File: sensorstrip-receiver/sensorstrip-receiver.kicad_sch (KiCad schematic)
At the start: 6 parts, among them J1 Conn_01x02_MountingPin, J2 Conn_01x02_MountingPin

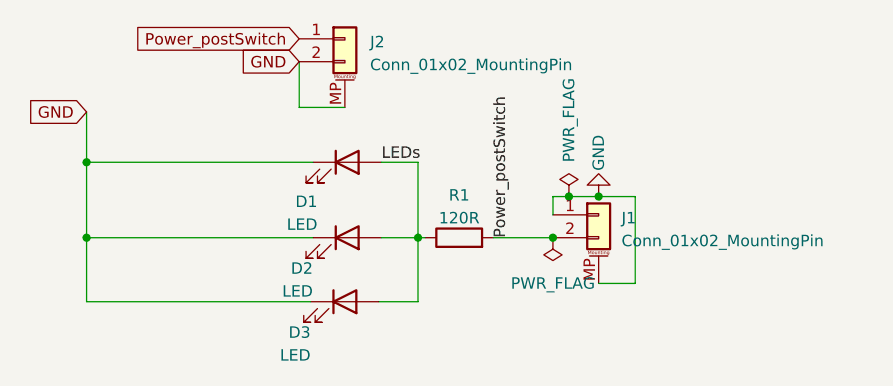
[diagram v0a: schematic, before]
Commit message: fix humongous oversight
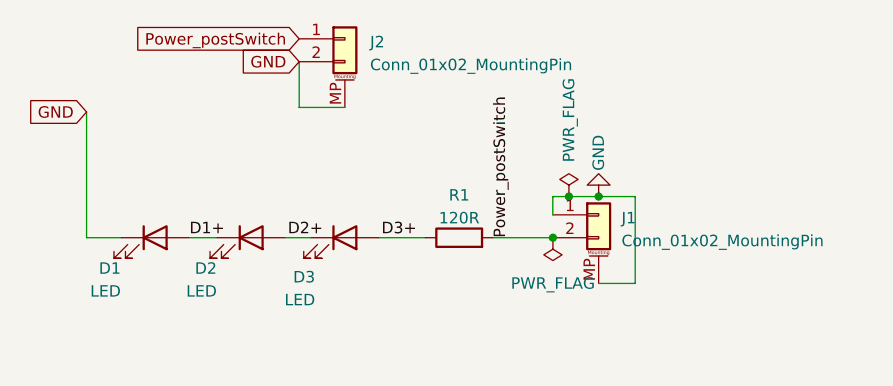
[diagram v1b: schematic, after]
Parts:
- renumbered D3 to D1, D1 to D3
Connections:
- net GND: no longer D2.1 (K), D3.1 (K)
- net LEDs renamed D3+
- net D3+: no longer D1.2 (A), D2.2 (A)
- new net D1+: D1.2 (A), D2.1 (K)
- new net D2+: D2.2 (A), D3.1 (K)
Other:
- moved on the sheet: D1, D2, D3
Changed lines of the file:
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@@
   (junction (at 117.348 86.868) (diameter 0) (color 0 0 0 0)
   )
-  (junction (at 63.754 83.058) (diameter 0) (color 0 0 0 0)
-  )
-  (junction (at 100.584 91.44) (diameter 0) (color 0 0 0 0)
-  )
-  (junction (at 63.754 91.44) (diameter 0) (color 0 0 0 0)
-  )
   (junction (at 120.65 86.868) (diameter 0) (color 0 0 0 0)
   )
   (junction (at 115.57 91.44) (diameter 0) (color 0 0 0 0)
   )
-  (wire (pts (xy 88.9 91.44) (xy 63.754 91.44))
-    (stroke (width 0) (type default) (color 0 0 0 0))
-  )
-  (wire (pts (xy 63.754 83.058) (xy 63.754 77.47))
-    (stroke (width 0) (type default) (color 0 0 0 0))
-  )
-  (wire (pts (xy 100.584 98.552) (xy 96.266 98.552))
+  (wire (pts (xy 78.232 91.44) (xy 75.184 91.44))
     (stroke (width 0) (type default) (color 0 0 0 0))
   )
@@
     (stroke (width 0) (type default) (color 0 0 0 0))
   )
-  (wire (pts (xy 63.754 91.44) (xy 63.754 98.552))
-    (stroke (width 0) (type default) (color 0 0 0 0))
-  )
   (wire (pts (xy 120.65 86.868) (xy 117.348 86.868))
     (stroke (width 0) (type default) (color 0 0 0 0))
@@
     (stroke (width 0) (type default) (color 0 0 0 0))
   )
-  (wire (pts (xy 101.346 91.44) (xy 100.584 91.44))
-    (stroke (width 0) (type default) (color 0 0 0 0))
-  )
-  (wire (pts (xy 88.646 98.552) (xy 63.754 98.552))
-    (stroke (width 0) (type default) (color 0 0 0 0))
-  )
-  (wire (pts (xy 63.754 83.058) (xy 63.754 91.44))
-    (stroke (width 0) (type default) (color 0 0 0 0))
-  )
-  (wire (pts (xy 100.584 83.058) (xy 96.52 83.058))
-    (stroke (width 0) (type default) (color 0 0 0 0))
-  )
-  (wire (pts (xy 100.584 91.44) (xy 100.584 83.058))
+  (wire (pts (xy 67.564 91.44) (xy 63.754 91.44))
+    (stroke (width 0) (type default) (color 0 0 0 0))
+  )
+  (wire (pts (xy 63.754 77.47) (xy 63.754 91.44))
+    (stroke (width 0) (type default) (color 0 0 0 0))
+  )
+  (wire (pts (xy 88.646 91.44) (xy 85.852 91.44))
     (stroke (width 0) (type default) (color 0 0 0 0))
   )
@@
     (stroke (width 0) (type default) (color 0 0 0 0))
   )
-  (wire (pts (xy 88.9 83.058) (xy 63.754 83.058))
-    (stroke (width 0) (type default) (color 0 0 0 0))
-  )
   (wire (pts (xy 115.57 86.868) (xy 115.57 88.9))
     (stroke (width 0) (type default) (color 0 0 0 0))
   )
-  (wire (pts (xy 100.584 91.44) (xy 100.584 98.552))
-    (stroke (width 0) (type default) (color 0 0 0 0))
-  )
-  (wire (pts (xy 100.584 91.44) (xy 96.52 91.44))
+  (wire (pts (xy 96.266 91.44) (xy 101.346 91.44))
     (stroke (width 0) (type default) (color 0 0 0 0))
   )
@@
     (effects (font (size 1.27 1.27)) (justify left bottom))
   )
-  (label "LEDs" (at 96.52 83.058 0)
+  (label "D2+" (at 86.106 91.44 0)
+    (effects (font (size 1.27 1.27)) (justify left bottom))
+  )
+  (label "D3+" (at 96.52 91.44 0)
+    (effects (font (size 1.27 1.27)) (justify left bottom))
+  )
+  (label "D1+" (at 75.184 91.44 0)
     (effects (font (size 1.27 1.27)) (justify left bottom))
   )
@@
     )
   )
-  (symbol (lib_id "Device:LED") (at 92.456 98.552 0) (unit 1)
-    (in_bom yes) (on_board yes)
-    (property "Reference" "D3" (id 0) (at 88.646 101.9718 0)
-      (effects (font (size 1.27 1.27)) (justify right))
-    )
-    (property "Value" "LED" (id 1) (at 88.646 104.5087 0)
-      (effects (font (size 1.27 1.27)) (justify right))
-    )
-    (property "Footprint" "sensorstrip:LED_THT-1.27mm-OrthogonalSMDAndTHT" (id 2) (at 92.456 98.552 0)
-      (effects (font (size 1.27 1.27)) hide)
-    )
-    (property "Datasheet" "~" (id 3) (at 92.456 98.552 0)
+  (symbol (lib_id "Device:LED") (at 71.374 91.44 0) (unit 1)
+    (in_bom yes) (on_board yes)
+    (property "Reference" "D1" (id 0) (at 67.564 94.8598 0)
+      (effects (font (size 1.27 1.27)) (justify right))
+    )
+    (property "Value" "LED" (id 1) (at 67.564 97.3967 0)
+      (effects (font (size 1.27 1.27)) (justify right))
+    )
+    (property "Footprint" "sensorstrip:LED_THT-1.27mm-OrthogonalSMDAndTHT" (id 2) (at 71.374 91.44 0)
+      (effects (font (size 1.27 1.27)) hide)
+    )
+    (property "Datasheet" "~" (id 3) (at 71.374 91.44 0)
       (effects (font (size 1.27 1.27)) hide)
     )
@@
     (pin "MP")
   )
-  (symbol (lib_id "Device:LED") (at 92.71 91.44 0) (unit 1)
-    (in_bom yes) (on_board yes)
-    (property "Reference" "D2" (id 0) (at 88.9 94.8598 0)
-      (effects (font (size 1.27 1.27)) (justify right))
-    )
-    (property "Value" "LED" (id 1) (at 88.9 97.3967 0)
-      (effects (font (size 1.27 1.27)) (justify right))
-    )
-    (property "Footprint" "sensorstrip:LED_THT-1.27mm-OrthogonalSMDAndTHT" (id 2) (at 92.71 91.44 0)
-      (effects (font (size 1.27 1.27)) hide)
-    )
-    (property "Datasheet" "~" (id 3) (at 92.71 91.44 0)
+  (symbol (lib_id "Device:LED") (at 82.042 91.44 0) (unit 1)
+    (in_bom yes) (on_board yes)
+    (property "Reference" "D2" (id 0) (at 78.232 94.8598 0)
+      (effects (font (size 1.27 1.27)) (justify right))
+    )
+    (property "Value" "LED" (id 1) (at 78.232 97.3967 0)
+      (effects (font (size 1.27 1.27)) (justify right))
+    )
+    (property "Footprint" "sensorstrip:LED_THT-1.27mm-OrthogonalSMDAndTHT" (id 2) (at 82.042 91.44 0)
+      (effects (font (size 1.27 1.27)) hide)
+    )
+    (property "Datasheet" "~" (id 3) (at 82.042 91.44 0)
       (effects (font (size 1.27 1.27)) hide)
     )
@@
     (pin "1")
   )
-  (symbol (lib_id "Device:LED") (at 92.71 83.058 0) (unit 1)
-    (in_bom yes) (on_board yes)
-    (property "Reference" "D1" (id 0) (at 89.408 87.4394 0)
-      (effects (font (size 1.27 1.27)) (justify right))
-    )
-    (property "Value" "LED" (id 1) (at 89.408 89.9794 0)
-      (effects (font (size 1.27 1.27)) (justify right))
-    )
-    (property "Footprint" "sensorstrip:LED_THT-1.27mm-OrthogonalSMDAndTHT" (id 2) (at 92.71 83.058 0)
-      (effects (font (size 1.27 1.27)) hide)
-    )
-    (property "Datasheet" "~" (id 3) (at 92.71 83.058 0)
+  (symbol (lib_id "Device:LED") (at 92.456 91.44 0) (unit 1)
+    (in_bom yes) (on_board yes)
+    (property "Reference" "D3" (id 0) (at 89.154 95.8214 0)
+      (effects (font (size 1.27 1.27)) (justify right))
+    )
+    (property "Value" "LED" (id 1) (at 89.154 98.3614 0)
+      (effects (font (size 1.27 1.27)) (justify right))
+    )
+    (property "Footprint" "sensorstrip:LED_THT-1.27mm-OrthogonalSMDAndTHT" (id 2) (at 92.456 91.44 0)
+      (effects (font (size 1.27 1.27)) hide)
+    )
+    (property "Datasheet" "~" (id 3) (at 92.456 91.44 0)
       (effects (font (size 1.27 1.27)) hide)
     )
@@
       (reference "#PWR0101") (unit 1) (value "GND") (footprint "")
     )
-    (path "/cb16ca99-563a-4e3e-999e-31e3640245a2"
+    (path "/0ddf7455-9149-4dbc-979b-f086dbd57a6e"
       (reference "D1") (unit 1) (value "LED") (footprint "sensorstrip:LED_THT-1.27mm-OrthogonalSMDAndTHT")
     )
@@
       (reference "D2") (unit 1) (value "LED") (footprint "sensorstrip:LED_THT-1.27mm-OrthogonalSMDAndTHT")
     )
-    (path "/0ddf7455-9149-4dbc-979b-f086dbd57a6e"
+    (path "/cb16ca99-563a-4e3e-999e-31e3640245a2"
       (reference "D3") (unit 1) (value "LED") (footprint "sensorstrip:LED_THT-1.27mm-OrthogonalSMDAndTHT")
     )
